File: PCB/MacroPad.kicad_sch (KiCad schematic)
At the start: 34 parts, among them M1 XIAO-RP2040, SW1 RotaryEncoder_Switch, SW10 SW_Push_45deg, SW11 SW_Push_45deg, SW12 SW_Push_45deg, SW13 SW_Push_45deg, SW14 SW_Push_45deg, SW15 SW_Push_45deg, SW16 SW_Push_45deg, SW17 SW_Push_45deg, SW2 SW_Push_45deg, SW3 SW_Push_45deg, SW4 SW_Push_45deg, SW5 SW_Push_45deg, SW6 SW_Push_45deg, SW7 SW_Push_45deg, SW8 SW_Push_45deg, SW9 SW_Push_45deg

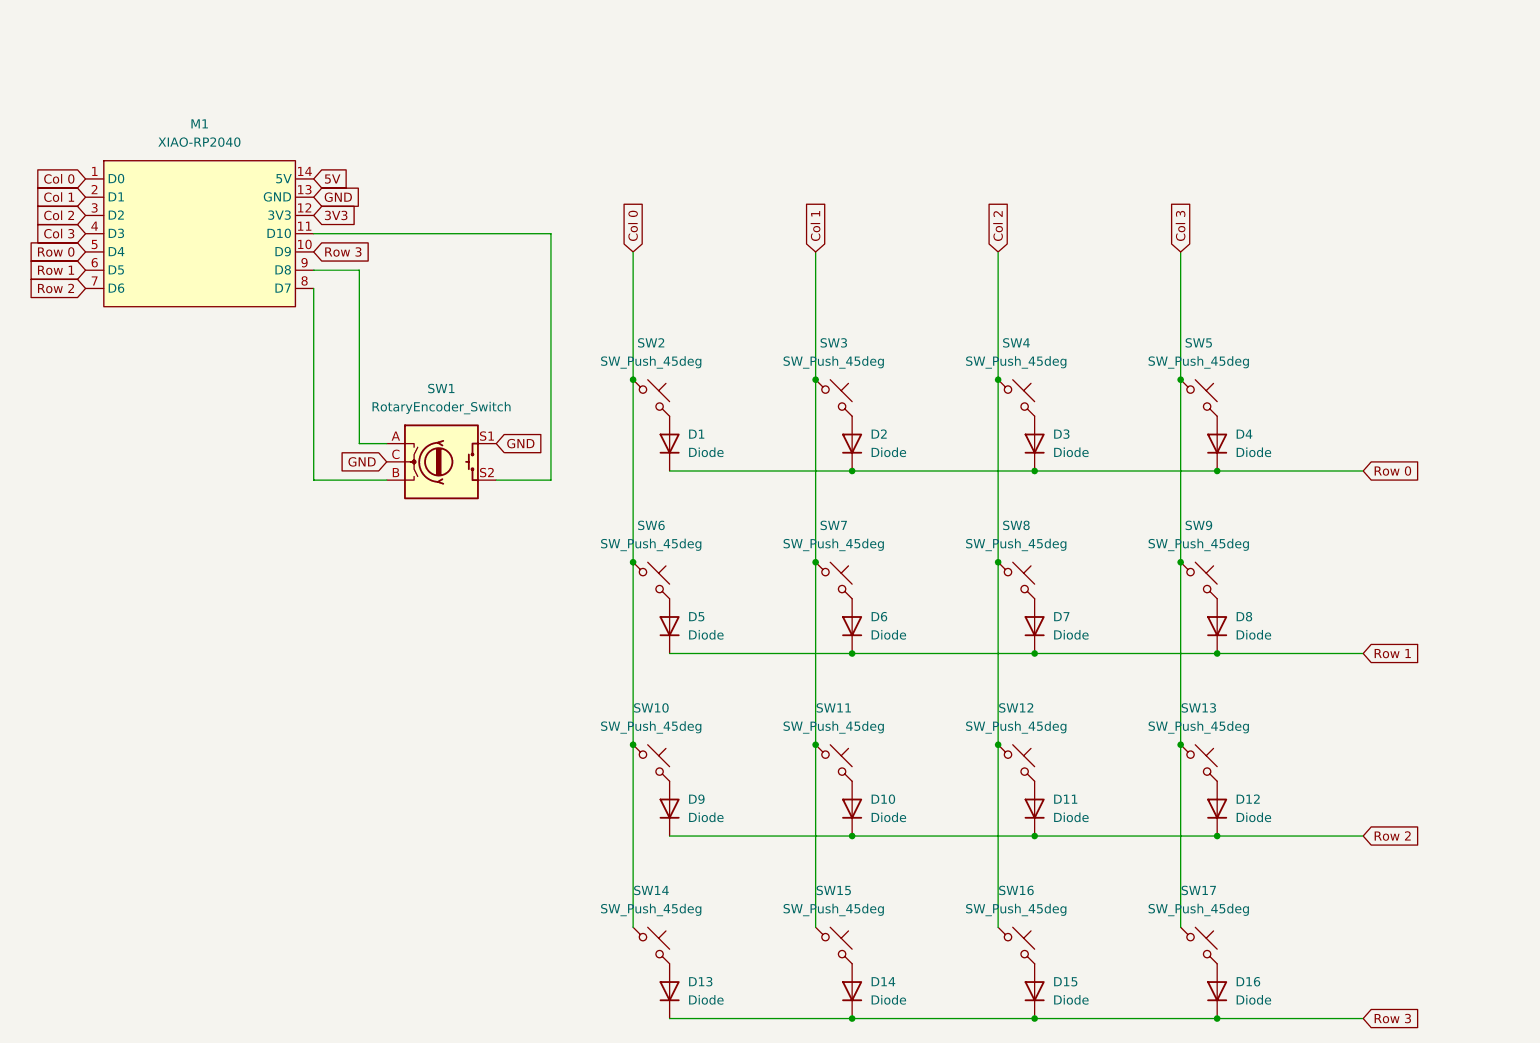
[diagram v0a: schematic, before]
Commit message: Routed and finished PCB
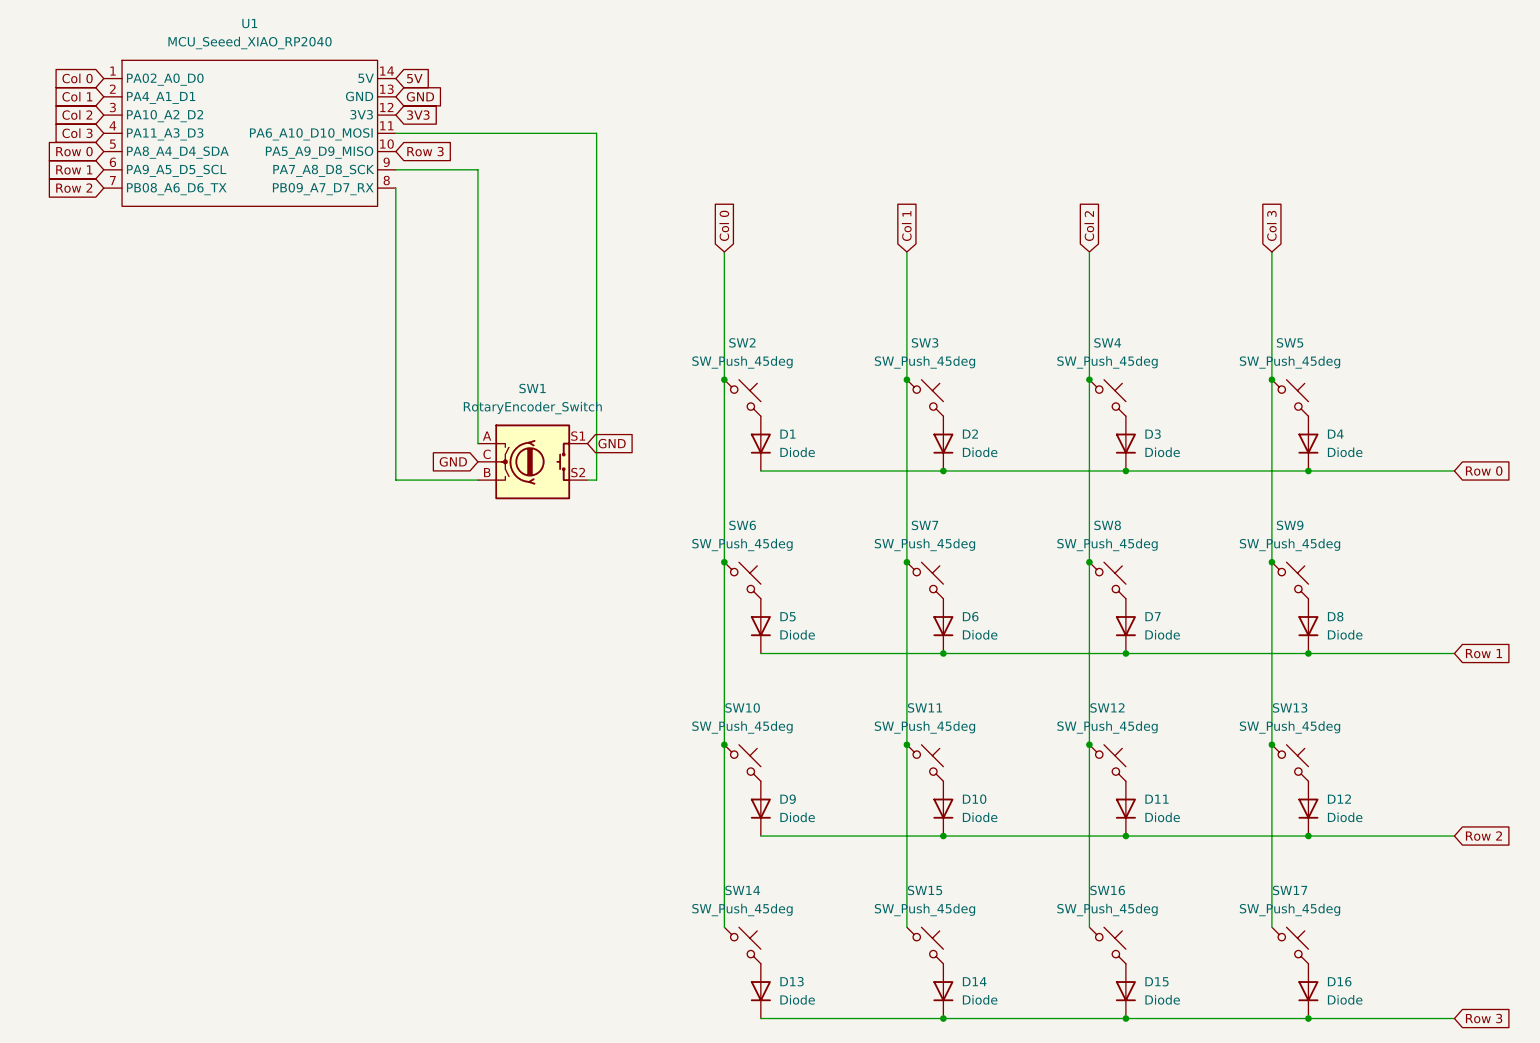
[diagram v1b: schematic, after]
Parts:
- removed M1: XIAO-RP2040, ScottoKeebs_MCU:Seeed_XIAO_RP2040, symbol xiao-rp2040:XIAO-RP2040
- added U1: MCU_Seeed_XIAO_RP2040, ScottoKeebs_MCU:Seeed_XIAO_RP2040, symbol ScottoKeebs:MCU_Seeed_XIAO_RP2040
- D1, D10, D11, D12, D13, D14, D15, D16, D2, D3, D4, D5, D6, D7, D8, D9: footprint Diode_THT:D_DO-35_SOD27_P7.62mm_Horizontal -> ScottoKeebs_Components:Diode_DO-35
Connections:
- net 3V3: now also U1.12 (3V3)
- net 5V: now also U1.14 (5V)
- net Col 0: now also U1.1 (PA02_A0_D0)
- net Col 1: now also U1.2 (PA4_A1_D1)
- net Col 2: now also U1.3 (PA10_A2_D2)
- net Col 3: now also U1.4 (PA11_A3_D3)
- net GND: now also U1.13 (GND)
- net Row 0: now also U1.5 (PA8_A4_D4_SDA)
- net Row 1: now also U1.6 (PA9_A5_D5_SCL)
- net Row 2: now also U1.7 (PB08_A6_D6_TX)
- net Row 3: now also U1.10 (PA5_A9_D9_MISO)
- net at SW1.S2: now also U1.11 (PA6_A10_D10_MOSI)
- net at SW1.B: now also U1.8 (PB09_A7_D7_RX)
- net at SW1.A: now also U1.9 (PA7_A8_D8_SCK)
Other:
- moved on the sheet: D1, D10, D11, D12, D13, D14, D15, D16, D2, D3, D4, D5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
